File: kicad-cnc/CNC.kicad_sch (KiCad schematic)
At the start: 14 parts, among them J1 Conn_02x25_Odd_Even, J2 Conn_02x08_Odd_Even, J3 Conn_01x04, U1 74AHC595, U2 ESP32_DevKitC_V4, U3 74AHC595

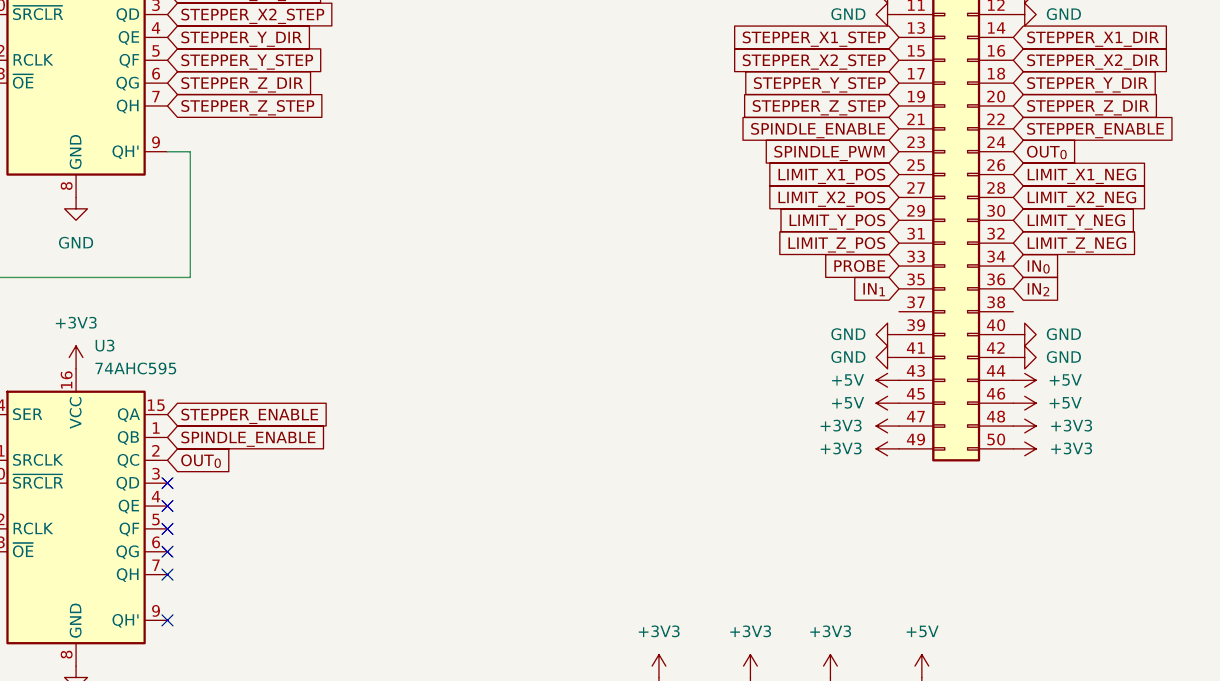
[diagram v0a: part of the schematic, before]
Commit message: started with the base pcb
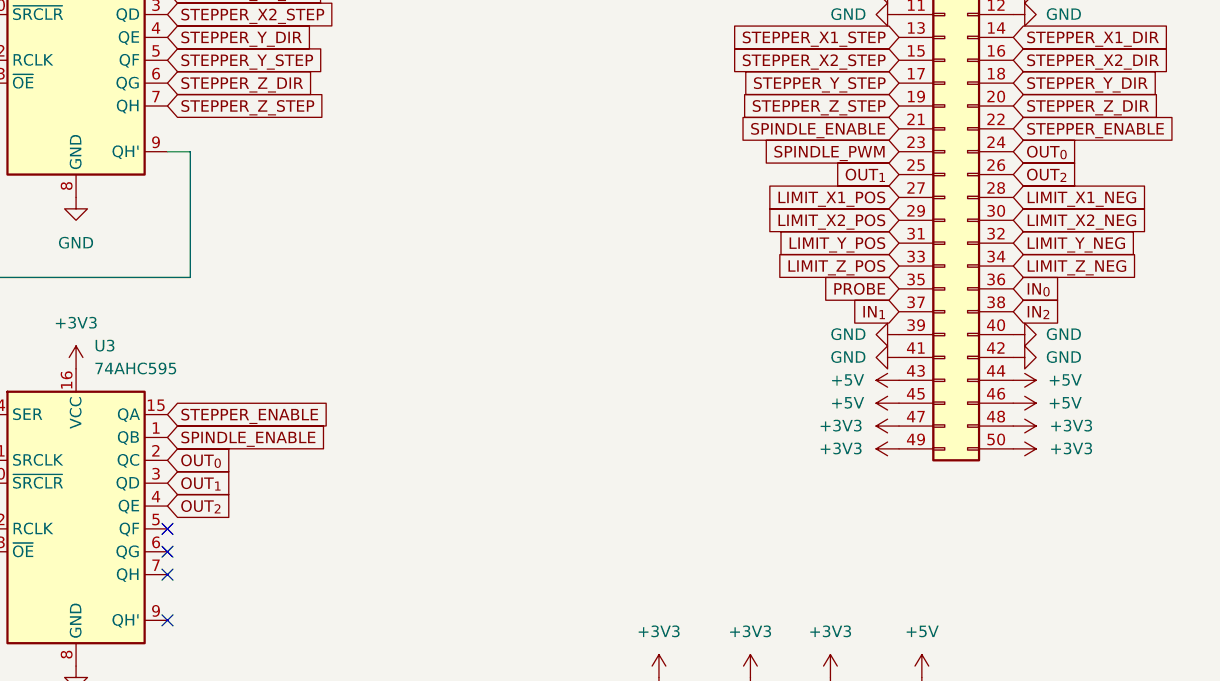
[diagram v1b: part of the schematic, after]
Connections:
- net IN_{0}: now also J1.36 (Pin_36); no longer J1.34 (Pin_34)
- net IN_{1}: now also J1.37 (Pin_37); no longer J1.35 (Pin_35)
- net IN_{2}: now also J1.38 (Pin_38); no longer J1.36 (Pin_36)
- net LIMIT_X1_NEG: now also J1.28 (Pin_28); no longer J1.26 (Pin_26)
- net LIMIT_X1_POS: now also J1.27 (Pin_27); no longer J1.25 (Pin_25)
- net LIMIT_X2_NEG: now also J1.30 (Pin_30); no longer J1.28 (Pin_28)
- net LIMIT_X2_POS: now also J1.29 (Pin_29); no longer J1.27 (Pin_27)
- net LIMIT_Y_NEG: now also J1.32 (Pin_32); no longer J1.30 (Pin_30)
- net LIMIT_Y_POS: now also J1.31 (Pin_31); no longer J1.29 (Pin_29)
- net LIMIT_Z_NEG: now also J1.34 (Pin_34); no longer J1.32 (Pin_32)
- net LIMIT_Z_POS: now also J1.33 (Pin_33); no longer J1.31 (Pin_31)
- net PROBE: now also J1.35 (Pin_35); no longer J1.33 (Pin_33)
- net OUT_{1}: now reaches U3.3 (QD)
- net OUT_{1}: now also J1.25 (Pin_25)
- net OUT_{2}: now reaches U3.4 (QE)
- net OUT_{2}: now also J1.26 (Pin_26)
- no-connect marks 16 -> 14
